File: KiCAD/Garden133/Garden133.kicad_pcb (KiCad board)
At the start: 4 copper layers, 66 x 39.4 mm, 46 parts, among them J1 USB_B_Micro, J2 Edge2x6_Connector, Q1 FS8205A, Q2 AO3401A, U1 SHTC3, U2 RFM95W-915S2, U3 ESP32-WROOM-32, U4 NCP114ASN330T1G, U5 DW01A, U6 TP4056

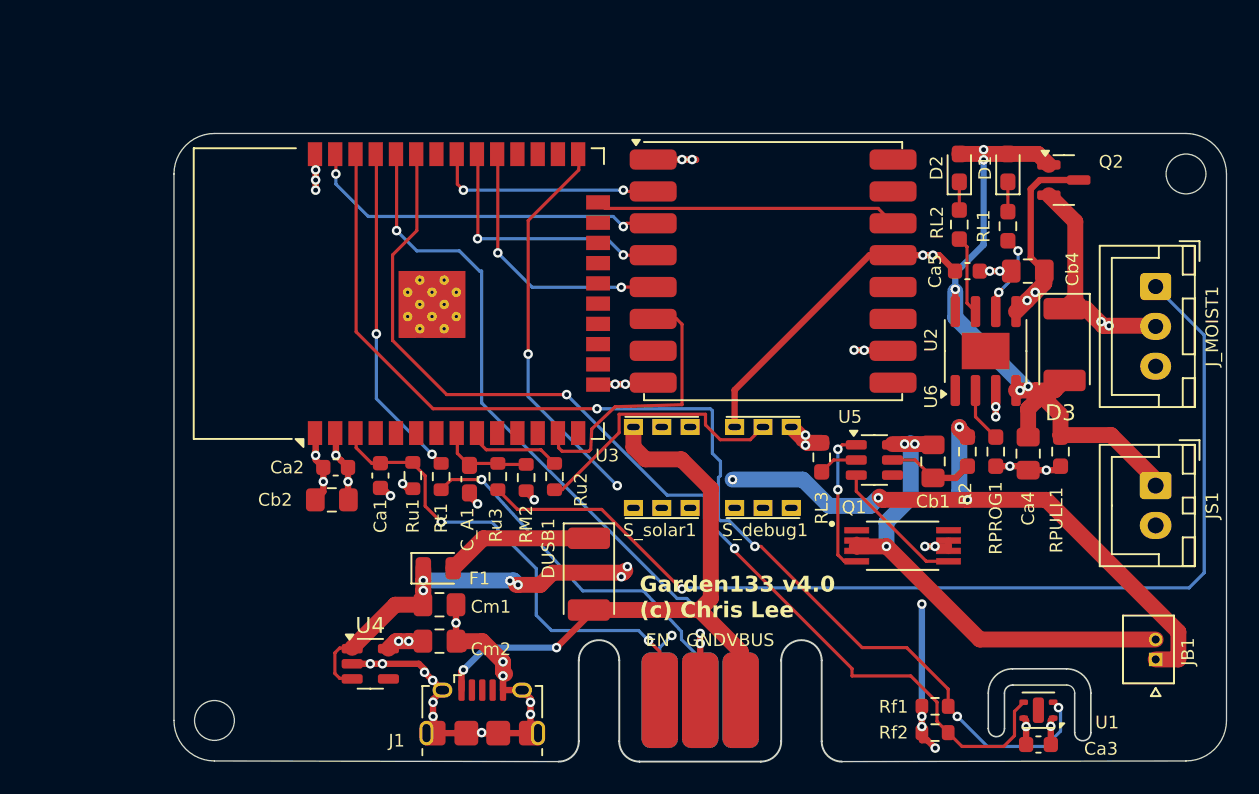
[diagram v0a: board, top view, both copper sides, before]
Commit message: Board version 5
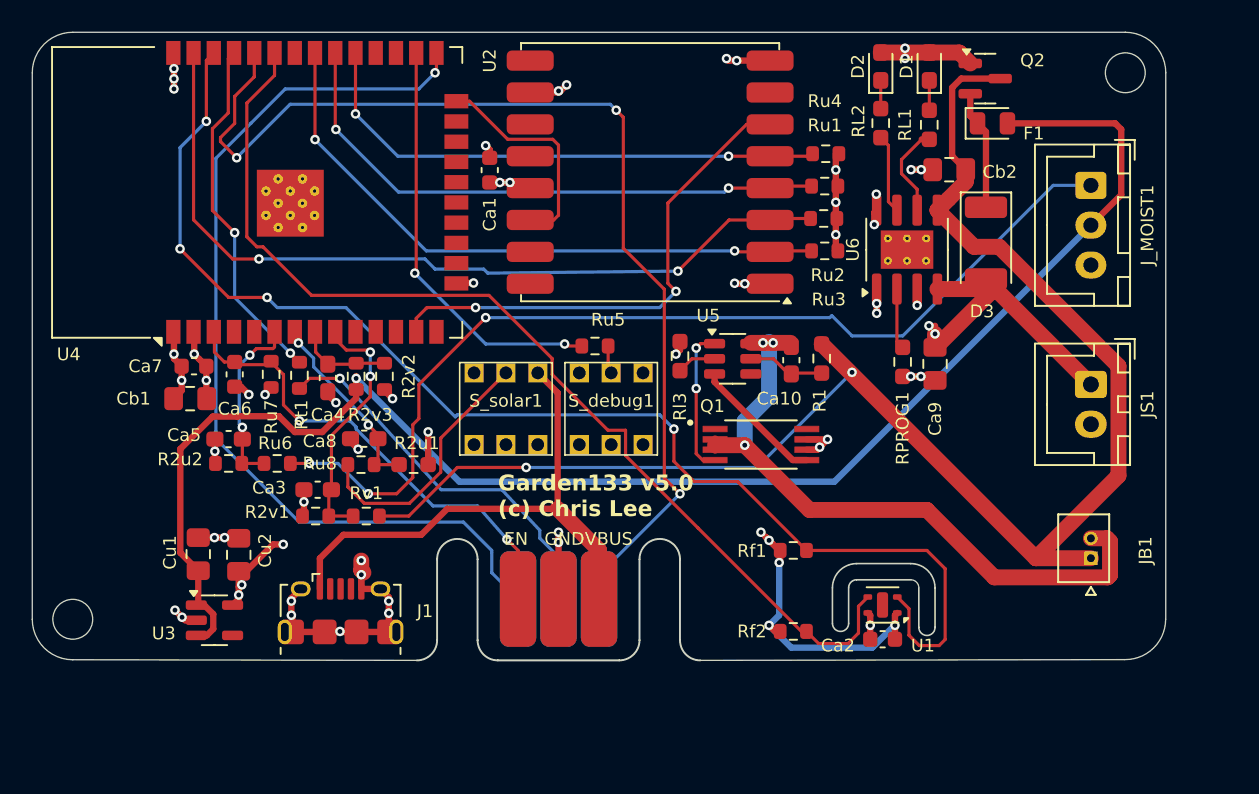
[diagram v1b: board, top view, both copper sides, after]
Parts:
- removed DUSB1: SS14, Diode_SMD:D_2010_5025Metric
- removed the REF** at (31.8, 63.5)
- removed the REF** at (92.7, 29.2)
- added Ca3: 100nF, Capacitor_SMD:C_0603_1608Metric_Pad1.08x0.95mm_HandSolder, F.Cu at (38.2, 49.0)
- added Ca5: 100nF, Capacitor_SMD:C_0603_1608Metric_Pad1.08x0.95mm_HandSolder, F.Cu at (32.6, 45.8)
- added Ca8: 100nF, Capacitor_SMD:C_0603_1608Metric_Pad1.08x0.95mm_HandSolder, F.Cu at (41.1, 45.8)
- added R2u2: 20k, Resistor_SMD:R_0603_1608Metric, F.Cu at (32.6, 47.4)
- added R2v1: 200k, Resistor_SMD:R_0603_1608Metric, F.Cu at (38.1, 50.7)
- added R2v3: 200k, Resistor_SMD:R_0603_1608Metric, F.Cu at (40.6, 41.9)
- added REF**: MountingHole_2.5mm_stencil_hole, chl33_library:MountingHole_2.5mm_stencil_hole, F.Cu at (88.9, 22.9)
- added REF**: MountingHole_2.5mm_stencil_hole, chl33_library:MountingHole_2.5mm_stencil_hole, F.Cu at (22.9, 57.1)
- added Ru1: 10k, Resistor_SMD:R_0603_1608Metric, F.Cu at (70.0, 30.0)
- added Ru2: 10k, Resistor_SMD:R_0603_1608Metric, F.Cu at (70.0, 32.0)
- added Ru4: 10k, Resistor_SMD:R_0603_1608Metric, F.Cu at (70.1, 27.9)
- added Ru6: 10k, Resistor_SMD:R_0603_1608Metric, F.Cu at (35.7, 47.4)
- added Ru8: 10k, Resistor_SMD:R_0603_1608Metric, F.Cu at (40.9, 47.4)
- added Rv1: 100k, Resistor_SMD:R_0603_1608Metric, F.Cu at (41.3, 50.7)
- Ca10: renamed from Cb1; value 10uF -> 100nF; footprint Capacitor_SMD:C_0805_2012Metric_Pad1.18x1.45mm_HandSolder -> Capacitor_SMD:C_0603_1608Metric_Pad1.08x0.95mm_HandSolder
- R2v2: renamed from RM2; value 20k -> 200k
- S_debug1: value BlueToggle -> SW_DPDT; footprint chl33_library:BlueToggle -> AliExpressSwitch:SW_SPDT_5.8x5.8_locking
- S_solar1: value BlueToggle -> SW_DPDY; footprint chl33_library:BlueToggle -> AliExpressSwitch:SW_SPDT_5.8x5.8_locking
- U6: footprint Package_SO:SOIC-8-1EP_3.9x4.9mm_P1.27mm_EP2.29x3mm -> Package_SO:SOIC-8-1EP_3.9x4.9mm_P1.27mm_EP2.41x3.3mm_ThermalVias
- moved F1 44.6 mm to (80.6, 26.0)
- moved R2u1 40.6 mm to (44.2, 47.4), turned to 180 degrees
- moved Ca1 30.6 mm to (49.0, 29.0), turned to -90 degrees
- moved Ru3 24.9 mm to (70.0, 34.0), turned to 0 degrees
- moved Cu1 15.5 mm to (30.7, 53.1), turned to 90 degrees
- moved Cu2 13.7 mm to (33.3, 53.1), turned to 90 degrees
- moved Rf1 13.2 mm to (68.1, 52.8)
- moved U1 11.8 mm to (73.7, 56.3)
- moved Ca2 11.8 mm to (73.7, 58.4)
- moved Ca6 11.1 mm to (33.0, 41.8)
- moved Ca10 10.9 mm to (67.9, 40.9)
- moved Ca4 10.9 mm to (38.9, 42.0)
- moved Ca7 10.9 mm to (30.5, 41.3)
- moved Q1 10.9 mm to (66.0, 46.2)
- moved R2v2 10.9 mm to (42.4, 41.9)
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- renumbered Ca5 to Ca1, Ca3 to Ca2, C_A1 to Ca4, Ca1 to Ca6, Ca2 to Ca7, Ca4 to Ca9, Cb2 to Cb1, Cb4 to Cb2, Cm1 to Cu1, Cm2 to Cu2, R2 to R1, RPULL1 to R2u1, RL3 to Rl3, Ru2 to Ru5, Ru1 to Ru7, U4 to U3, U3 to U4
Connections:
- D3 pad 1: +5V -> Net-(D3-K)
- F1 pad 1: +5V -> Net-(D3-K)
- F1 pad 2: Net-(DUSB1-K) -> +5V
- Q2 pad 2: +5V -> Net-(D3-K)
- R2u1 pad 1: VSOLAR+ -> GND
- R2u1 pad 2: GND -> ADC1_CH7
- Ru3 pad 1: ADC1_CH4 -> GPIO19
- Ru3 pad 2: AMOIST -> +3.3V
- Ru5 pad 1: GPIO33 -> GPIO26
- S_solar1 pad 2: VBATTERY+ -> VSOLAR+
- S_solar1 pad 4: GND -> unconnected-(S_solar1-A-Pad4)
- S_solar1 pad 5: GND -> unconnected-(S_solar1-B-Pad5)
- U4 pad 26: unconnected-(U3-IO4-Pad26) -> GPIO26
- U4 pad 6: unconnected-(U3-IO34-Pad6) -> ADC1_CH6
- U4 pad 7: unconnected-(U3-IO35-Pad7) -> ADC1_CH7
- U4 pad 9: GPIO33 -> ADC1_CH5
- U6 pad 1: unconnected-(U6-TEMP-Pad1) -> GND
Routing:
- net VSOLAR+: track 42.4 -> 91.0 mm, vias 5 -> 6
- net GPIO23: track 23.1 -> 52.1 mm
- net VBATTERY+: track 71.0 -> 97.6 mm, vias 6 -> 2
- net GPIO26: track 0.00 -> 26.2 mm, vias 0 -> 2
- net GPIO19: track 14.7 -> 39.4 mm
- net RX: track 45.2 -> 69.6 mm, vias 1 -> 3
- net GPIO18: track 16.8 -> 36.4 mm
- net GPIO0: track 40.5 -> 59.0 mm, vias 3 -> 1
- net GPIO5: track 16.9 -> 33.6 mm
- net ADC1_CH5: track 0.00 -> 15.9 mm, vias 0 -> 2
- net Net-(Ru5-Pad2): track 17.1 -> 1.77 mm
- net GPIO14: track 17.6 -> 32.5 mm, vias 0 -> 2
- net ADC1_CH7: track 0.00 -> 12.2 mm, vias 0 -> 2
- net ADC1_CH6: track 0.00 -> 11.3 mm, vias 0 -> 2
- net +5V: track 86.9 -> 97.9 mm, vias 8 -> 1
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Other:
- board size 66 x 39.4 mm -> 71.1 x 39.4 mm
- board text added: "Garden133 v5.0 (c) Chris Lee"
- board text removed: "Garden133 v4.0 (c) Chris Lee"
